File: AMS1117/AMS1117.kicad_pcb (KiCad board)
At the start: 2 copper layers, 5 parts, among them U1 AMS1117-3.3

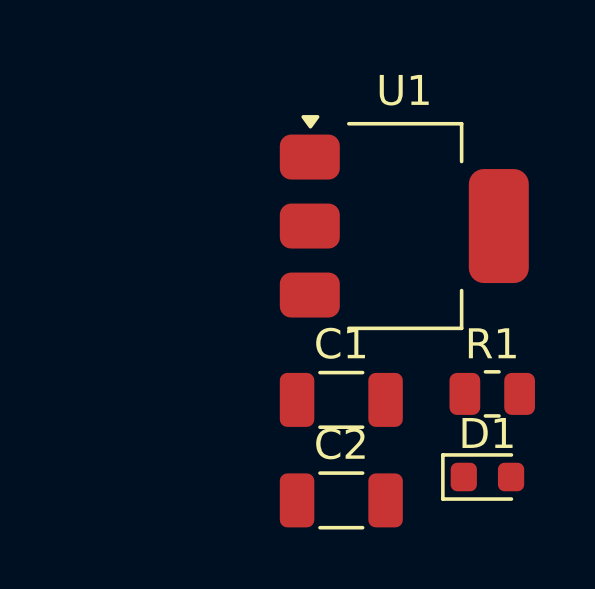
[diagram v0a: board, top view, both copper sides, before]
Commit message: added json source
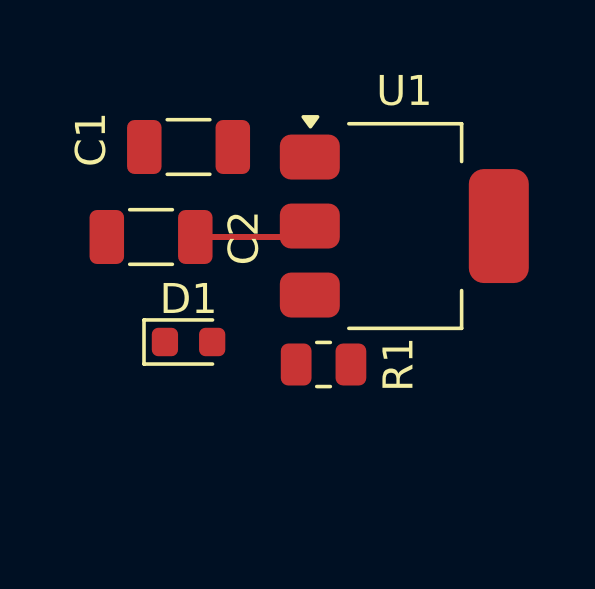
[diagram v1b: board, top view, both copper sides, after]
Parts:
- moved D1 10.9 mm to (123.2, 79.8)
- moved C2 10.8 mm to (122.0, 76.2), turned to 180 degrees
- moved C1 9.85 mm to (123.2, 73.2)
- moved R1 5.71 mm to (127.8, 80.5)
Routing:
- net /LDO_3V3_AMS1117_/3V3: track 0.00 -> 3.97 mm
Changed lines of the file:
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@@
 	(footprint "Capacitor_SMD:C_1206_3216Metric"
 		(layer "F.Cu")
-		(at 128.3425 81.68)
+		(at 123.25 73.25)
 		(descr "Capacitor SMD 1206 (3216 Metric), square (rectangular) end terminal, IPC_7351 nominal, (Body size source: IPC-SM-782 page 76, https://www.pcb-3d.com/wordpress/wp-content/uploads/ipc-sm-782a_amendment_1_and_2.pdf), generated with kicad-footprint-generator")
 		(tags "capacitor")
 		(property "Reference" "C1"
-			(at 0 -1.85 0)
+			(at -3.25 -0.25 90)
 			(layer "F.SilkS")
 			(effects
@@
 	(footprint "Resistor_SMD:R_0805_2012Metric"
 		(layer "F.Cu")
-		(at 133.3725 81.48)
+		(at 127.75 80.5)
 		(descr "Resistor SMD 0805 (2012 Metric), square (rectangular) end terminal, IPC_7351 nominal, (Body size source: IPC-SM-782 page 72, https://www.pcb-3d.com/wordpress/wp-content/uploads/ipc-sm-782a_amendment_1_and_2.pdf), generated with kicad-footprint-generator")
 		(tags "resistor")
 		(property "Reference" "R1"
-			(at 0 -1.65 0)
+			(at 2.5 0 -90)
 			(layer "F.SilkS")
 			(effects
@@
 	(footprint "LED_SMD:LED_0603_1608Metric"
 		(layer "F.Cu")
-		(at 133.2125 84.25)
+		(at 123.25 79.75)
 		(descr "LED SMD 0603 (1608 Metric), square (rectangular) end terminal, IPC_7351 nominal, (Body size source: http://www.tortai-tech.com/upload/download/2011102023233369053.pdf), generated with kicad-footprint-generator")
 		(tags "LED")
@@
 	(footprint "Capacitor_SMD:C_1206_3216Metric"
 		(layer "F.Cu")
-		(at 128.3425 85.03)
+		(at 122 76.25 180)
 		(descr "Capacitor SMD 1206 (3216 Metric), square (rectangular) end terminal, IPC_7351 nominal, (Body size source: IPC-SM-782 page 76, https://www.pcb-3d.com/wordpress/wp-content/uploads/ipc-sm-782a_amendment_1_and_2.pdf), generated with kicad-footprint-generator")
 		(tags "capacitor")
 		(property "Reference" "C2"
-			(at 0 -1.85 0)
+			(at -3.0925 -0.03 90)
 			(layer "F.SilkS")
 			(effects
@@
 		)
 		(property "Value" "22uF/10V"
-			(at 0 1.85 0)
+			(at 0 1.850001 360)
 			(layer "F.Fab")
 			(effects
@@
 		)
 		(property "Footprint" "Capacitor_SMD:C_1206_3216Metric"
-			(at 0 0 0)
+			(at 0 0 180)
 			(unlocked yes)
 			(layer "F.Fab")
@@
 		)
 		(property "Datasheet" ""
-			(at 0 0 0)
+			(at 0 0 180)
 			(unlocked yes)
 			(layer "F.Fab")
@@
 		)
 		(property "Description" ""
-			(at 0 0 0)
+			(at 0 0 180)
 			(unlocked yes)
 			(layer "F.Fab")
@@
 		)
 		(property "LCSC Part #" ""
-			(at 0 0 0)
+			(at 0 0 180)
 			(unlocked yes)
 			(layer "F.Fab")
@@
 		(attr smd)
 		(fp_line
+			(start -0.711252 0.91)
+			(end 0.711252 0.91)
+			(stroke
+				(width 0.12)
+				(type solid)
+			)
+			(layer "F.SilkS")
+		)
+		(fp_line
 			(start -0.711252 -0.91)
 			(end 0.711252 -0.91)
@@
 		)
 		(fp_line
-			(start -0.711252 0.91)
-			(end 0.711252 0.91)
-			(stroke
-				(width 0.12)
-				(type solid)
-			)
-			(layer "F.SilkS")
+			(start 2.3 1.15)
+			(end -2.3 1.15)
+			(stroke
+				(width 0.05)
+				(type solid)
+			)
+			(layer "F.CrtYd")
+		)
+		(fp_line
+			(start 2.3 -1.15)
+			(end 2.3 1.15)
+			(stroke
+				(width 0.05)
+				(type solid)
+			)
+			(layer "F.CrtYd")
+		)
+		(fp_line
+			(start -2.3 1.15)
+			(end -2.3 -1.15)
+			(stroke
+				(width 0.05)
+				(type solid)
+			)
+			(layer "F.CrtYd")
 		)
 		(fp_line
@@
 		)
 		(fp_line
-			(start -2.3 1.15)
-			(end -2.3 -1.15)
-			(stroke
-				(width 0.05)
-				(type solid)
-			)
-			(layer "F.CrtYd")
-		)
-		(fp_line
-			(start 2.3 -1.15)
-			(end 2.3 1.15)
-			(stroke
-				(width 0.05)
-				(type solid)
-			)
-			(layer "F.CrtYd")
-		)
-		(fp_line
-			(start 2.3 1.15)
-			(end -2.3 1.15)
-			(stroke
-				(width 0.05)
-				(type solid)
-			)
-			(layer "F.CrtYd")
+			(start 1.6 0.8)
+			(end -1.6 0.8)
+			(stroke
+				(width 0.1)
+				(type solid)
+			)
+			(layer "F.Fab")
+		)
+		(fp_line
+			(start 1.6 -0.8)
+			(end 1.6 0.8)
+			(stroke
+				(width 0.1)
+				(type solid)
+			)
+			(layer "F.Fab")
+		)
+		(fp_line
+			(start -1.6 0.8)
+			(end -1.6 -0.8)
+			(stroke
+				(width 0.1)
+				(type solid)
+			)
+			(layer "F.Fab")
 		)
 		(fp_line
@@
 			(layer "F.Fab")
 		)
-		(fp_line
-			(start -1.6 0.8)
-			(end -1.6 -0.8)
-			(stroke
-				(width 0.1)
-				(type solid)
-			)
-			(layer "F.Fab")
-		)
-		(fp_line
-			(start 1.6 -0.8)
-			(end 1.6 0.8)
-			(stroke
-				(width 0.1)
-				(type solid)
-			)
-			(layer "F.Fab")
-		)
-		(fp_line
-			(start 1.6 0.8)
-			(end -1.6 0.8)
-			(stroke
-				(width 0.1)
-				(type solid)
-			)
-			(layer "F.Fab")
-		)
 		(fp_text user "${REFERENCE}"
-			(at 0 0 0)
+			(at 0 0 360)
 			(layer "F.Fab")
 			(effects
@@
 		)
 		(pad "1" smd roundrect
-			(at -1.475 0)
+			(at -1.475001 0 180)
 			(size 1.15 1.8)
 			(layers "F.Cu" "F.Paste" "F.Mask")
@@
 		)
 		(pad "2" smd roundrect
-			(at 1.475 0)
+			(at 1.475001 0 180)
 			(size 1.15 1.8)
 			(layers "F.Cu" "F.Paste" "F.Mask")
@@
 	)
 	(gr_rect
-		(start 124 70.75)
-		(end 137.5 88.5)
+		(start 118.75 70.375)
+		(end 135.25 81.875)
 		(stroke
 			(width 0.1)
@@
 		(layer "Dwgs.User")
 	)
+	(segment
+		(start 126.9275 76.25)
+		(end 127.2925 75.885)
+		(width 0.2)
+		(layer "F.Cu")
+		(net 3)
+	)
+	(segment
+		(start 123.475001 76.25)
+		(end 126.9275 76.25)
+		(width 0.2)
+		(layer "F.Cu")
+		(net 3)
+	)
 )
